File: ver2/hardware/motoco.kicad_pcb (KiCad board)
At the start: 2 copper layers, 102 parts, among them IC1 TLE7182EM, IC2 TLE4269G, M1 Motor_DC, Q1 BC846B

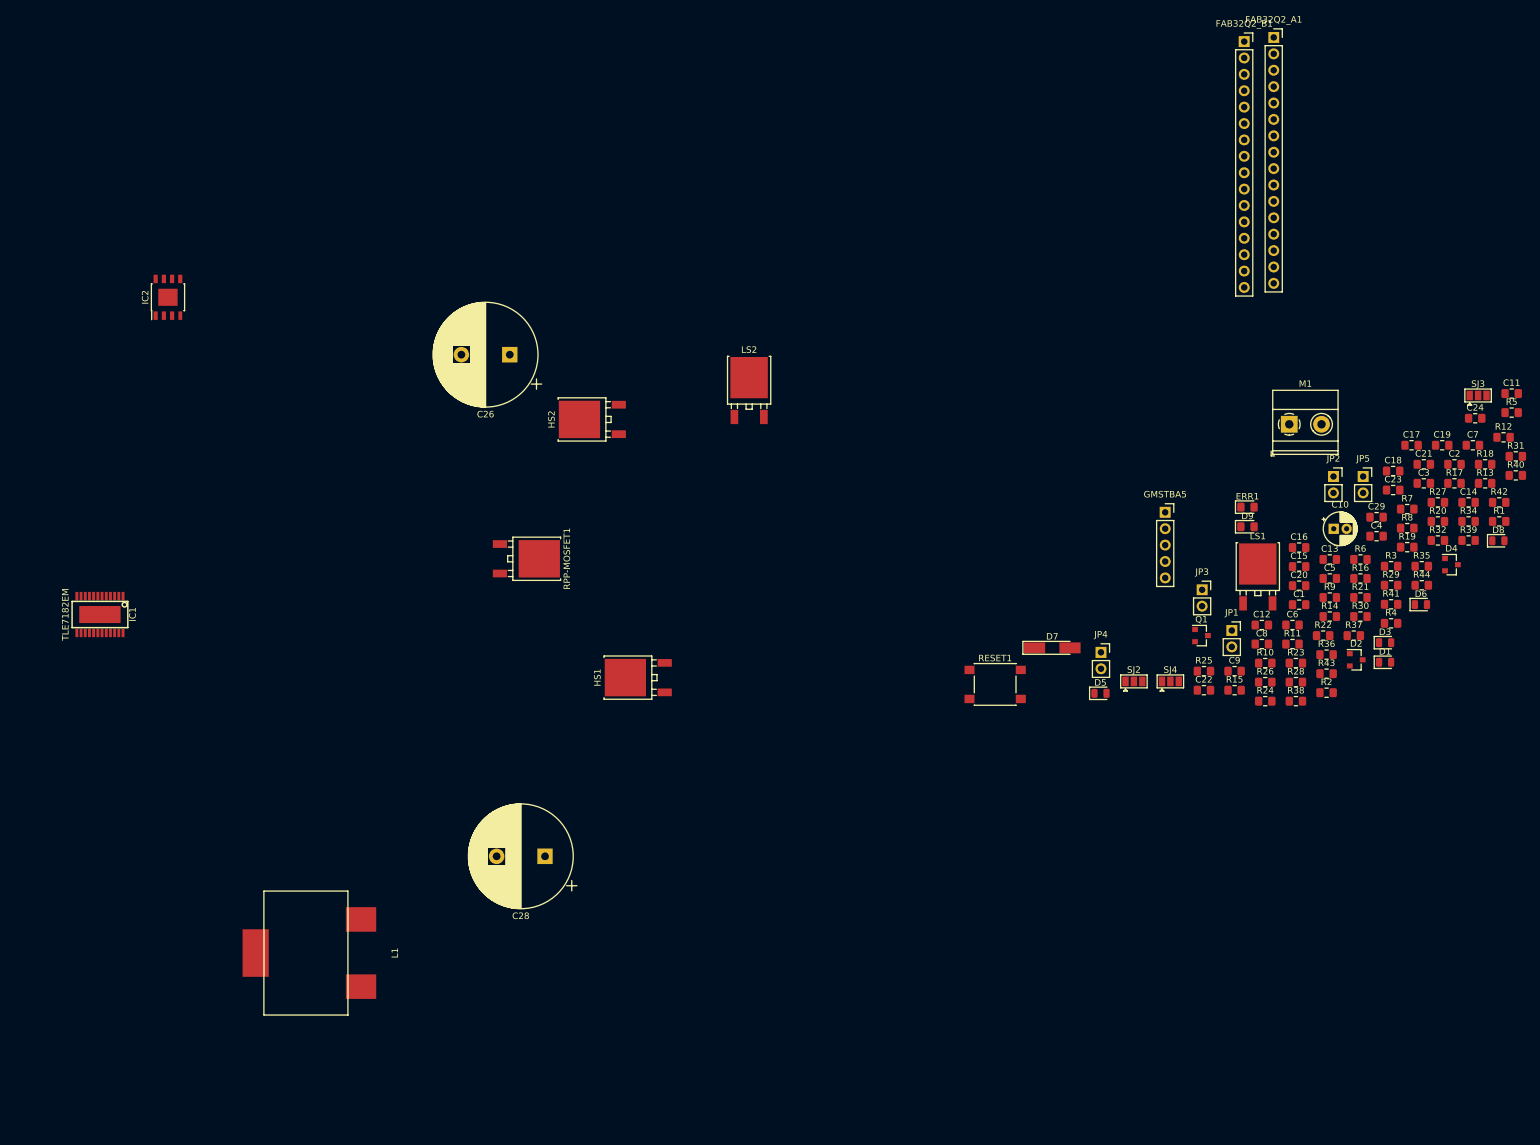
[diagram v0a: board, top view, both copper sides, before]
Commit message: update
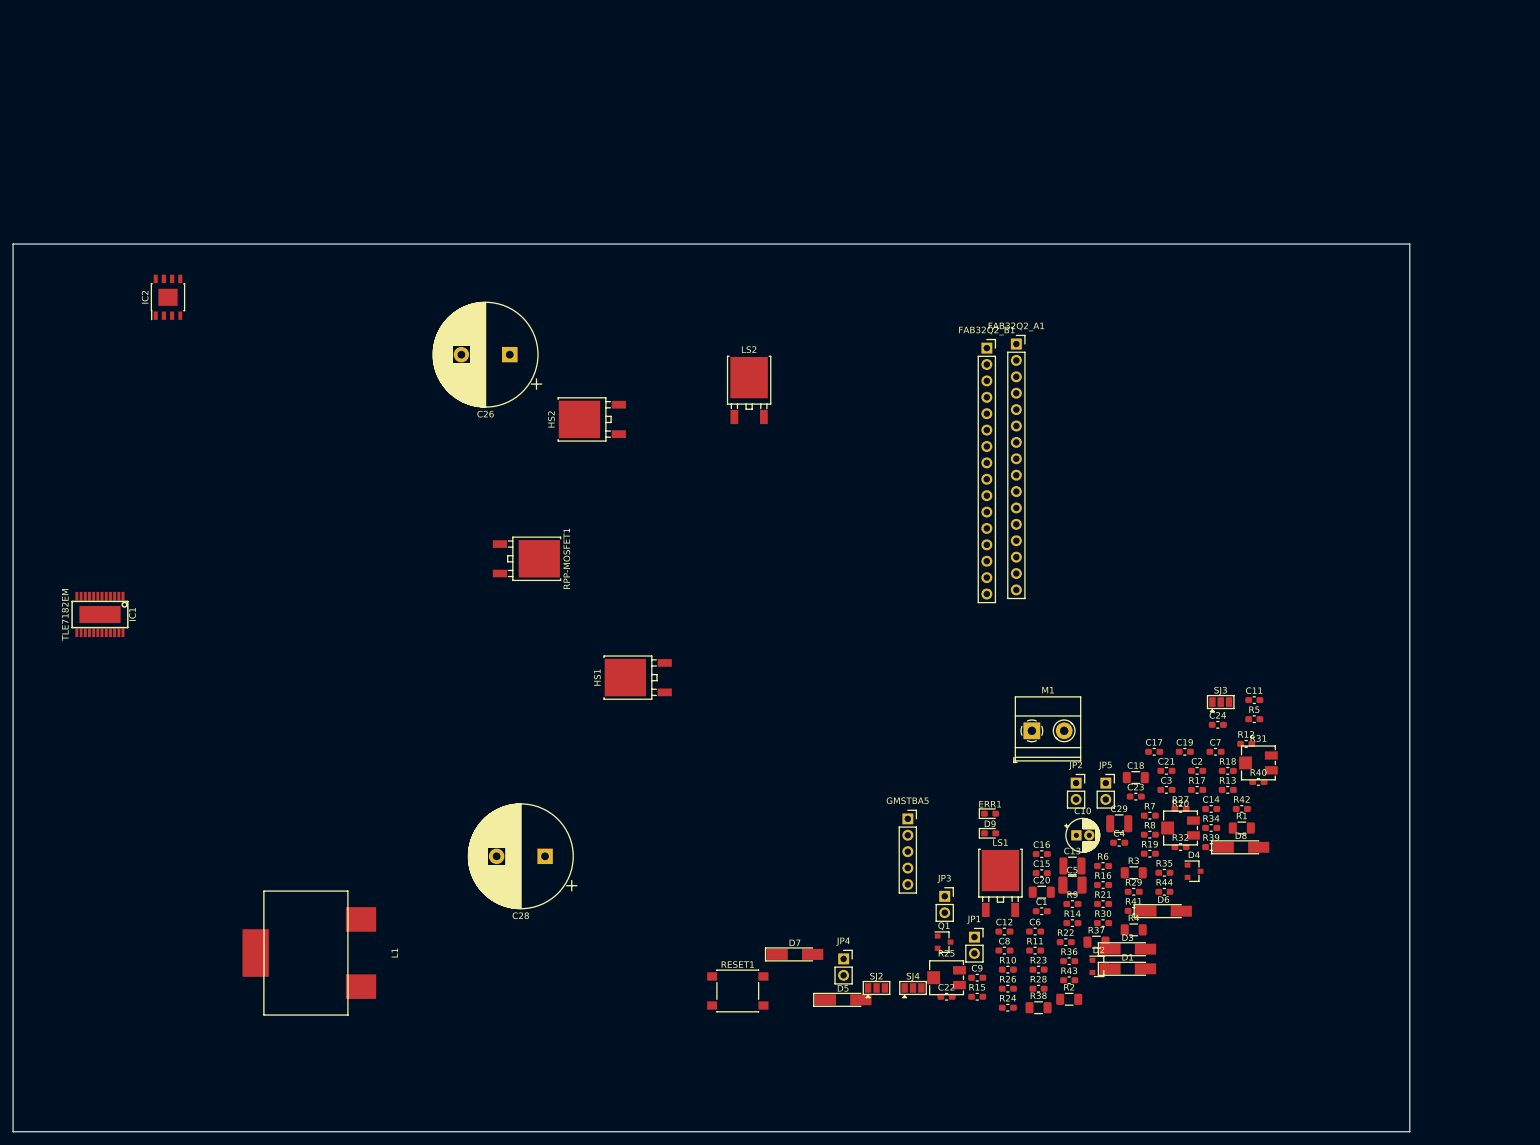
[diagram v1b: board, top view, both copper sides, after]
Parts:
- C1, C11, C12, C14, C15, C16, C17, C19, C2, C21, C22, C23, C24, C3, C4, C6, C7, C8, C9: footprint Capacitor_SMD:C_0805_2012Metric_Pad1.15x1.40mm_HandSolder -> Capacitor_SMD:C_0603_1608Metric_Pad1.05x0.95mm_HandSolder
- C13, C29: footprint Capacitor_SMD:C_0805_2012Metric_Pad1.15x1.40mm_HandSolder -> Capacitor_SMD:C_1210_3225Metric
- C18, C20: footprint Capacitor_SMD:C_0805_2012Metric_Pad1.15x1.40mm_HandSolder -> Capacitor_SMD:C_1206_3216Metric
- C5: footprint Capacitor_SMD:C_0805_2012Metric_Pad1.15x1.40mm_HandSolder -> Capacitor_SMD:C_1210_3225Metric_Pad1.42x2.65mm_HandSolder
- D1, D3, D5, D6, D8: footprint Diode_SMD:D_0805_2012Metric -> Diode_SMD:D_MiniMELF_Handsoldering
- D9, ERR1: footprint LED_SMD:LED_0805_2012Metric_Pad1.15x1.40mm_HandSolder -> LED_SMD:LED_0603_1608Metric_Pad1.05x0.95mm_HandSolder
- R1, R2, R3, R37, R38, R4: footprint Resistor_SMD:R_0805_2012Metric_Pad1.15x1.40mm_HandSolder -> Resistor_SMD:R_1206_3216Metric
- R10, R11, R12, R13, R14, R15, R16, R17, R18, R19, R21, R22, R23, R24, R26, R27, R28, R29, R30, R32, R34, R35, R36, R39, R40, R41, R42, R43, R44, R5, R6, R7, R8, R9: footprint Resistor_SMD:R_0805_2012Metric_Pad1.15x1.40mm_HandSolder -> Resistor_SMD:R_0603_1608Metric_Pad1.05x0.95mm_HandSolder
- R20, R25, R31: footprint Resistor_SMD:R_0805_2012Metric_Pad1.15x1.40mm_HandSolder -> Potentiometer_SMD:Potentiometer_Vishay_TS53YJ_Vertical
- moved R24 62.0 mm to (212.8, 150.6)
- moved R38 62.0 mm to (217.6, 150.6)
- moved C10 62.0 mm to (223.4, 123.9)
- moved C11 62.0 mm to (251.0, 102.9)
- moved C12 62.0 mm to (212.3, 138.8)
- moved C13 62.0 mm to (222.8, 128.6)
- moved C14 62.0 mm to (244.3, 119.8)
- moved C16 62.0 mm to (218.1, 126.8)
- moved C17 62.0 mm to (235.5, 110.9)
- moved C18 62.0 mm to (232.6, 114.9)
- moved C19 62.0 mm to (240.2, 110.9)
- moved C20 62.0 mm to (218.1, 132.7)
- moved C23 62.0 mm to (232.6, 117.9)
- moved C3 62.0 mm to (237.4, 116.8)
- moved C7 62.0 mm to (245.0, 110.9)
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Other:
- board outline added: 216.4 x 137.5 mm
